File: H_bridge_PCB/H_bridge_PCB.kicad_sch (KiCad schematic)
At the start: 15 parts, among them J1 PWR IN, J2 CH L, J3 CH R, J4 Bluetooth module connector, J5 PWR IN jumper, U1 DRV8844PWPR, U2 MC79M05_TO252

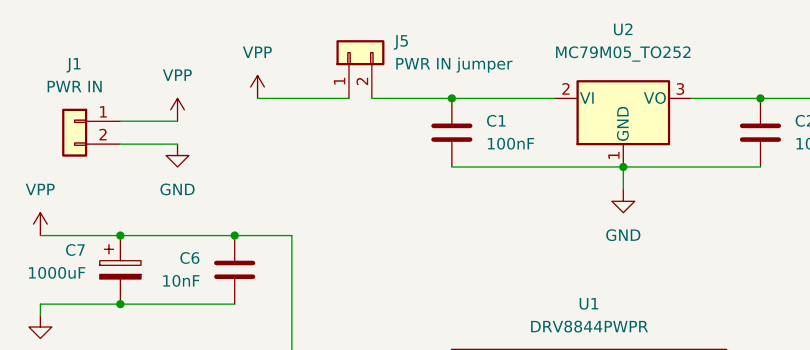
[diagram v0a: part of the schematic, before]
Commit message: yah
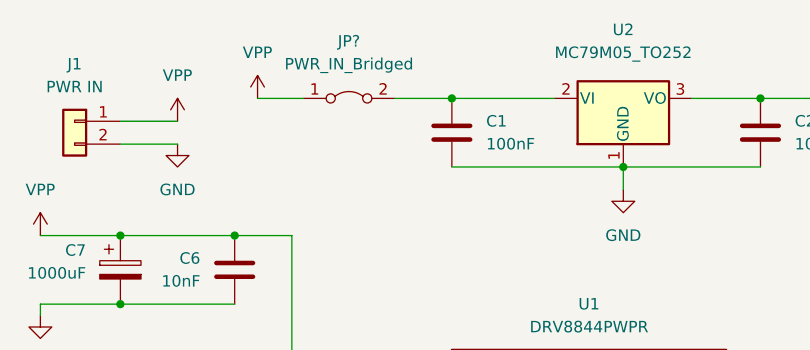
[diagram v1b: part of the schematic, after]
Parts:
- removed J5: PWR IN jumper, Connector_PinHeader_2.54mm:PinHeader_1x02_P2.54mm_Vertical, symbol Connector_Generic:Conn_01x02
- added JP?: PWR_IN_Bridged, Connector_PinHeader_2.54mm:PinHeader_1x02_P2.54mm_Vertical, symbol Jumper:Jumper_2_Bridged
- J4: footprint Connector_PinSocket_2.54mm:PinSocket_1x06_P2.54mm_Vertical -> Connector_PinSocket_2.54mm:PinSocket_1x06_P2.54mm_Horizontal
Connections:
- net VPP: now also JP?.1 (A)
- net at C1.1, U2.2 (VI): now also JP?.2 (B)
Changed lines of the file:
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@@
   (junction (at 160.02 106.68) (diameter 0) (color 0 0 0 0)
   )
+  (junction (at 133.35 73.66) (diameter 0) (color 0 0 0 0)
+  )
+  (junction (at 165.1 81.28) (diameter 0) (color 0 0 0 0)
+  )
   (junction (at 170.18 50.8) (diameter 0) (color 0 0 0 0)
   )
-  (junction (at 133.35 73.66) (diameter 0) (color 0 0 0 0)
-  )
-  (junction (at 165.1 81.28) (diameter 0) (color 0 0 0 0)
-  )
   (junction (at 133.35 66.04) (diameter 0) (color 0 0 0 0)
   )
@@
     (stroke (width 0) (type default) (color 0 0 0 0))
   )
+  (wire (pts (xy 163.83 50.8) (xy 170.18 50.8))
+    (stroke (width 0) (type default) (color 0 0 0 0))
+  )
   (wire (pts (xy 146.05 114.3) (xy 146.05 135.89))
     (stroke (width 0) (type default) (color 0 0 0 0))
@@
     (stroke (width 0) (type default) (color 0 0 0 0))
   )
+  (wire (pts (xy 148.59 50.8) (xy 153.67 50.8))
+    (stroke (width 0) (type default) (color 0 0 0 0))
+  )
   (wire (pts (xy 129.54 143.51) (xy 153.67 143.51))
     (stroke (width 0) (type default) (color 0 0 0 0))
@@
     (stroke (width 0) (type default) (color 0 0 0 0))
   )
-  (wire (pts (xy 148.59 50.8) (xy 158.75 50.8))
-    (stroke (width 0) (type default) (color 0 0 0 0))
-  )
   (wire (pts (xy 196.85 50.8) (xy 204.47 50.8))
     (stroke (width 0) (type default) (color 0 0 0 0))
@@
   )
   (wire (pts (xy 148.59 106.68) (xy 160.02 106.68))
-    (stroke (width 0) (type default) (color 0 0 0 0))
-  )
-  (wire (pts (xy 161.29 50.8) (xy 170.18 50.8))
     (stroke (width 0) (type default) (color 0 0 0 0))
   )
@@
     )
     (pin "1")
-  )
-  (symbol (lib_id "Connector_Generic:Conn_01x02") (at 158.75 45.72 90) (unit 1)
-    (in_bom yes) (on_board yes) (fields_autoplaced)
-    (property "Reference" "J5" (id 0) (at 163.83 44.4499 90)
-      (effects (font (size 1.27 1.27)) (justify right))
-    )
-    (property "Value" "PWR IN jumper" (id 1) (at 163.83 46.9899 90)
-      (effects (font (size 1.27 1.27)) (justify right))
-    )
-    (property "Footprint" "Connector_PinHeader_2.54mm:PinHeader_1x02_P2.54mm_Vertical" (id 2) (at 158.75 45.72 0)
-      (effects (font (size 1.27 1.27)) hide)
-    )
-    (property "Datasheet" "~" (id 3) (at 158.75 45.72 0)
-      (effects (font (size 1.27 1.27)) hide)
-    )
-    (pin "1")
-    (pin "2")
   )
   (symbol (lib_id "power:GND") (at 139.7 55.88 0) (unit 1)
@@
     (pin "1")
   )
+  (symbol (lib_id "Jumper:Jumper_2_Bridged") (at 158.75 50.8 0) (unit 1)
+    (in_bom yes) (on_board yes) (fields_autoplaced)
+    (property "Reference" "JP?" (id 0) (at 158.75 44.45 0))
+    (property "Value" "PWR_IN_Bridged" (id 1) (at 158.75 46.99 0))
+    (property "Footprint" "Connector_PinHeader_2.54mm:PinHeader_1x02_P2.54mm_Vertical" (id 2) (at 158.75 50.8 0)
+      (effects (font (size 1.27 1.27)) hide)
+    )
+    (property "Datasheet" "~" (id 3) (at 158.75 50.8 0)
+      (effects (font (size 1.27 1.27)) hide)
+    )
+    (pin "1")
+    (pin "2")
+  )
   (symbol (lib_id "power:VPP") (at 148.59 50.8 0) (unit 1)
     (in_bom yes) (on_board yes) (fields_autoplaced)
@@
     (property "Reference" "J4" (id 0) (at 40.64 99.06 0))
     (property "Value" "Bluetooth module connector" (id 1) (at 40.64 101.6 0))
-    (property "Footprint" "Connector_PinSocket_2.54mm:PinSocket_1x06_P2.54mm_Vertical" (id 2) (at 40.64 110.49 0)
+    (property "Footprint" "Connector_PinSocket_2.54mm:PinSocket_1x06_P2.54mm_Horizontal" (id 2) (at 40.64 110.49 0)
       (effects (font (size 1.27 1.27)) hide)
     )
@@
     )
     (path "/dc87c548-b2b5-4a9b-981c-35fe12ca10ac"
-      (reference "J4") (unit 1) (value "Bluetooth module connector") (footprint "Connector_PinSocket_2.54mm:PinSocket_1x06_P2.54mm_Vertical")
-    )
-    (path "/2d2db02e-f97c-4eea-85ad-75588a32c590"
-      (reference "J5") (unit 1) (value "PWR IN jumper") (footprint "Connector_PinHeader_2.54mm:PinHeader_1x02_P2.54mm_Vertical")
+      (reference "J4") (unit 1) (value "Bluetooth module connector") (footprint "Connector_PinSocket_2.54mm:PinSocket_1x06_P2.54mm_Horizontal")
+    )
+    (path "/46401a3d-3fbf-44e0-aed7-5f36da2d4da4"
+      (reference "JP?") (unit 1) (value "PWR_IN_Bridged") (footprint "Connector_PinHeader_2.54mm:PinHeader_1x02_P2.54mm_Vertical")
     )
     (path "/808f661a-faf0-48d4-9cfb-e2979be8a144"
